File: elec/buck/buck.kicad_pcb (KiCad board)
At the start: 2 copper layers, 33 x 27.9 mm, 14 parts, among them J1 Conn_01x08, J2 Conn_01x08

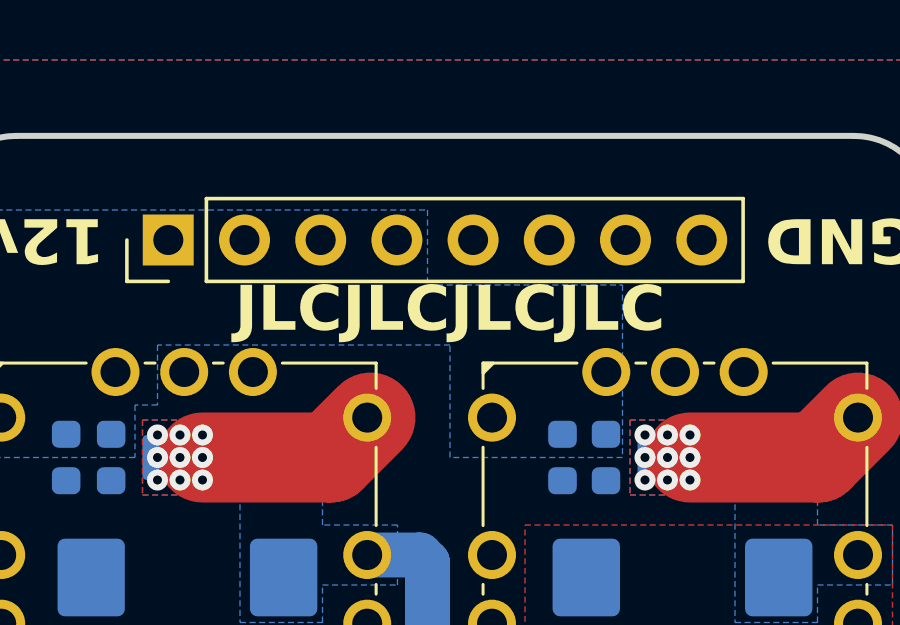
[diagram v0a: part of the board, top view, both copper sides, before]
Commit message: prod: prod
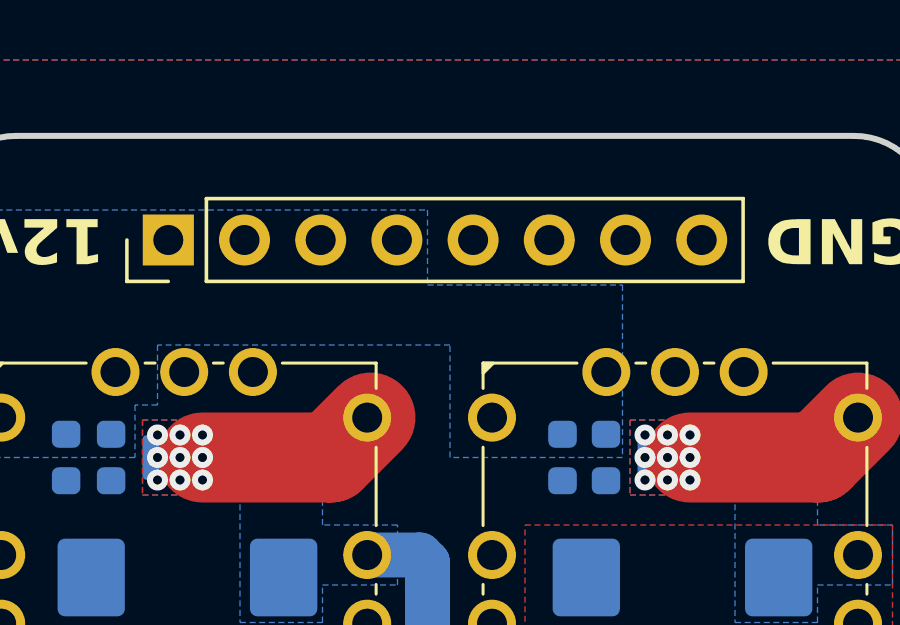
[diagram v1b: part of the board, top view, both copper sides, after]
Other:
- board text removed: "JLCJLCJLCJLC"
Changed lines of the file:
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@@
-		)
-	)
-	(gr_text "JLCJLCJLCJLC\n"
-		(at 105.01 102.979999 0)
-		(layer "F.SilkS")
-		(effects
-			(font
-				(size 1.5 1.5)
-				(thickness 0.3)
-				(bold yes)
-			)
 		)
 	)
